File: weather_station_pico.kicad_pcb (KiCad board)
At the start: 2 copper layers, 90.2 x 90.2 mm, 30 parts, among them J1 POWER, J2 WSPEED, J3 WDIR, J4 I2C, SW1 SW_Push, U1 LM7805_TO220, U2 E220-900T22D, U3 Pico, U4 74HC4051, U5 LM35-LP, U6 LM385BZ-1.2

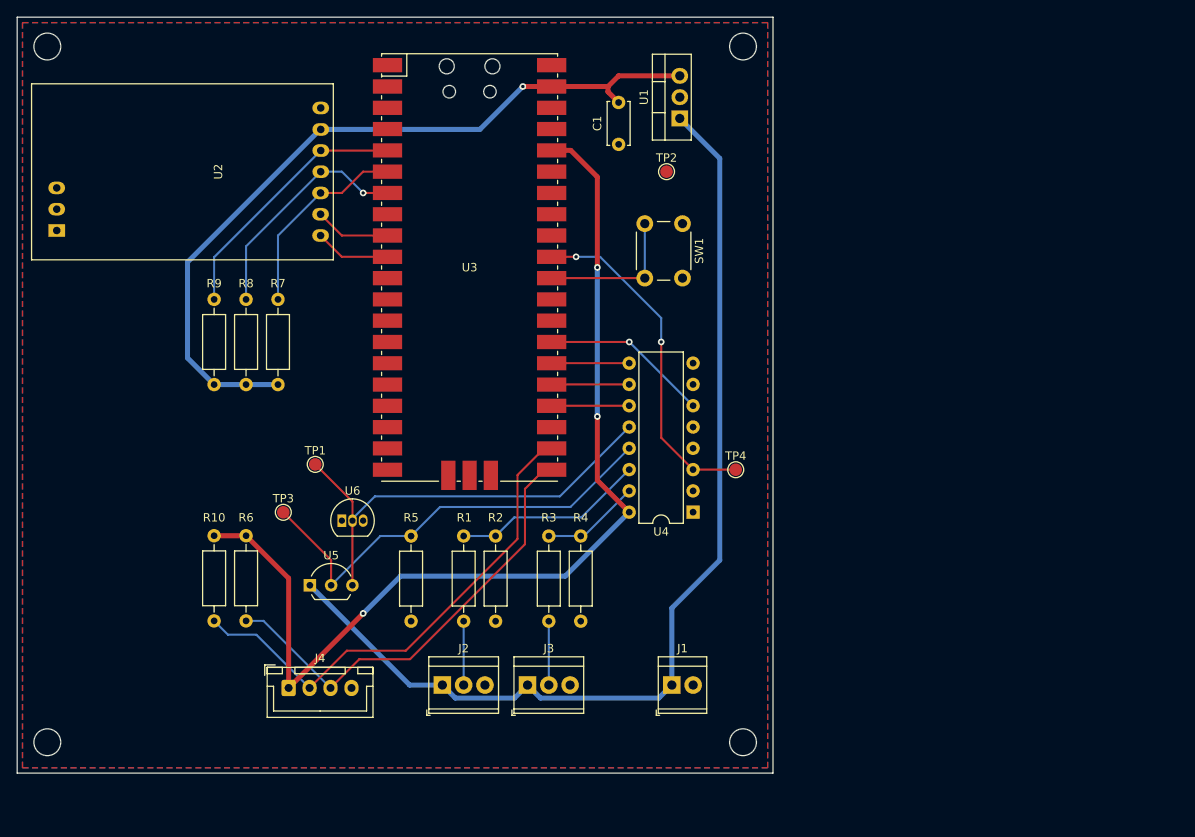
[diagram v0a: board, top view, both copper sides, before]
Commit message: ready for plot
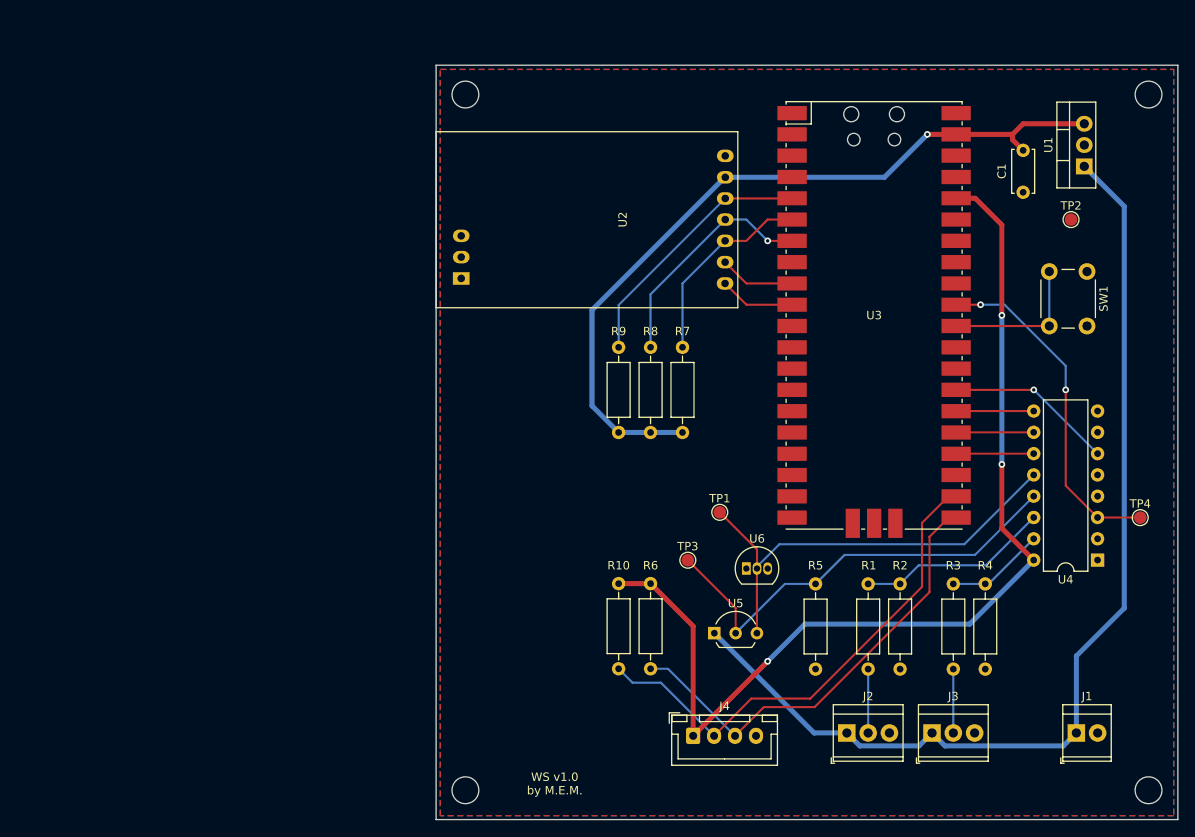
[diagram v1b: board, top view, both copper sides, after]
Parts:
- moved H3 50.2 mm to (118.9, 65.7)
- moved H4 50.2 mm to (118.9, 148.7)
- moved H1 48.7 mm to (200.4, 148.7)
- moved H2 48.7 mm to (200.4, 65.7)
- moved J1 48.6 mm to (191.8, 141.9)
- moved R4 48.6 mm to (180.9, 124.1)
- moved U4 48.6 mm to (194.3, 121.3)
- moved U5 48.6 mm to (148.6, 130.0)
- moved J3 48.6 mm to (174.6, 141.9)
- moved J4 48.6 mm to (146.1, 142.2)
- moved R1 48.6 mm to (166.9, 134.3)
- moved R2 48.6 mm to (170.7, 124.1)
- moved R5 48.6 mm to (160.7, 124.1)
- moved R6 48.6 mm to (141.0, 124.1)
- moved R7 48.6 mm to (144.8, 106.0)
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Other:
- board size 90.2 x 90.2 mm -> 88.5 x 90 mm
- board text added: "WS v1.0 by M.E.M."
